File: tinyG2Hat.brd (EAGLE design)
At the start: 102.6 x 69.1 mm, 31 parts

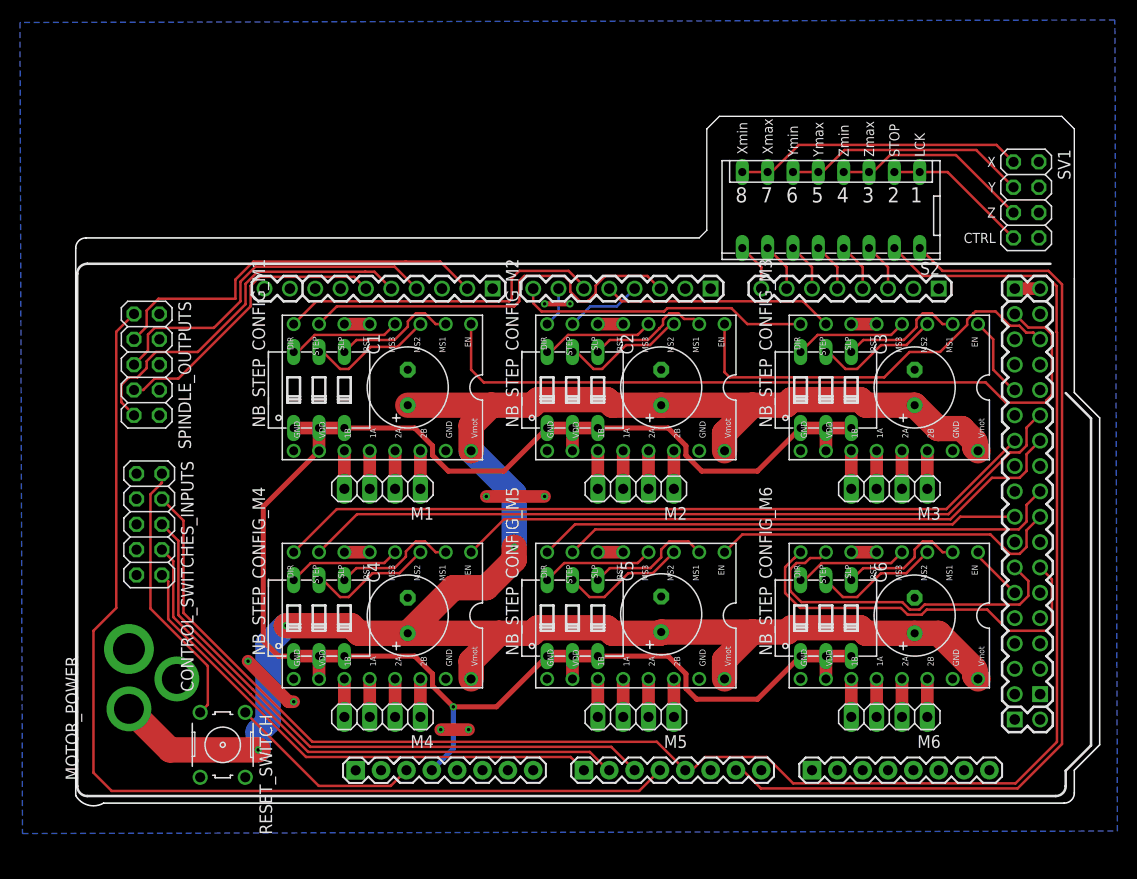
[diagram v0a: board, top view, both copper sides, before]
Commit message: Sérigraphie finie
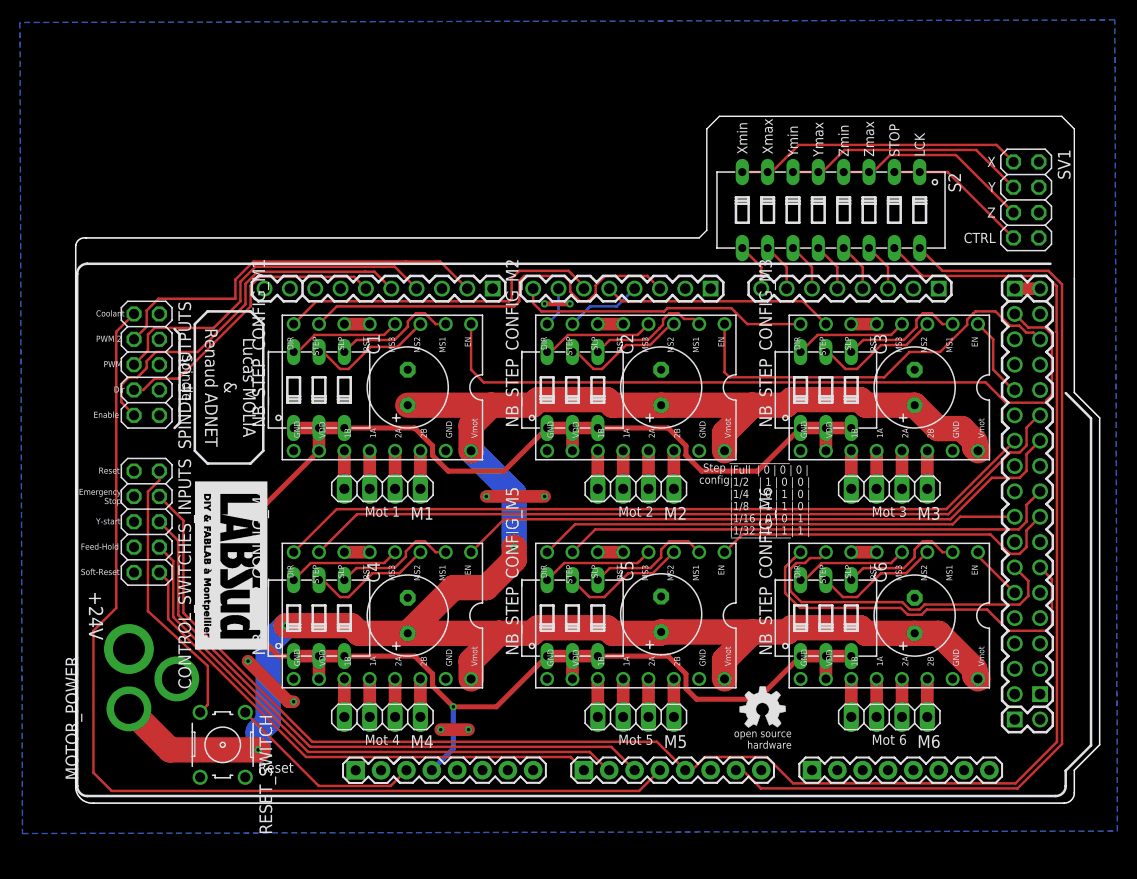
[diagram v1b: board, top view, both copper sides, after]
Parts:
- added U$7: (no value), Aliom:OPEN_HARDWARE_5MM
- added U$8: (no value), Aliom:LABSUD_15MM
- S2: device switch-dil:DP-08 -> switch-dil:DIP08YL
- moved CONTROL_SWITCHES_INPUTS 0.36 mm to (6.86, 28.4)
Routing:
- net N$50: track 27.1 -> 27.6 mm
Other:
- board size 102.6 x 69.1 mm -> 102.6 x 68.8 mm
- board text added: "+24V"
- board text added: "Coolant"
- board text added: "Dir"
- board text added: "Emergency Stop"
- board text added: "Enable"
- board text added: "Feed-Hold"
- board text added: "Lucas MOLIA & Renaud ADNET"
- board text added: "Mot 1"
- board text added: "Mot 2"
- board text added: "Mot 3"
- board text added: "Mot 4"
- board text added: "Mot 5"
- board text added: "Mot 6"
- board text added: "PWM"
- board text added: "PWM 2"
- board text added: "Reset"
- board text added: "Soft-Reset"
- board text added: "Spindle"
- board text added: "Step config"
- board text added: "Y-start"
- board text added: "____________"
- board text added: "____________ |Full | 0 | 0 | 0 | |1/2 | 1 | 0 | 0 | |1/4 | 0 | 1 | 0 | |1/8 | 1 | 1 | 0 | |1/16 | 0 | 0 | 1 | |1/32 | 1 | 1 | 1 |"
